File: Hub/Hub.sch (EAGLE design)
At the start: 16 parts, among them X1 C-GRID-04-15-91, X2 C-GRID-04-15-91, X3 C-GRID-04-15-91

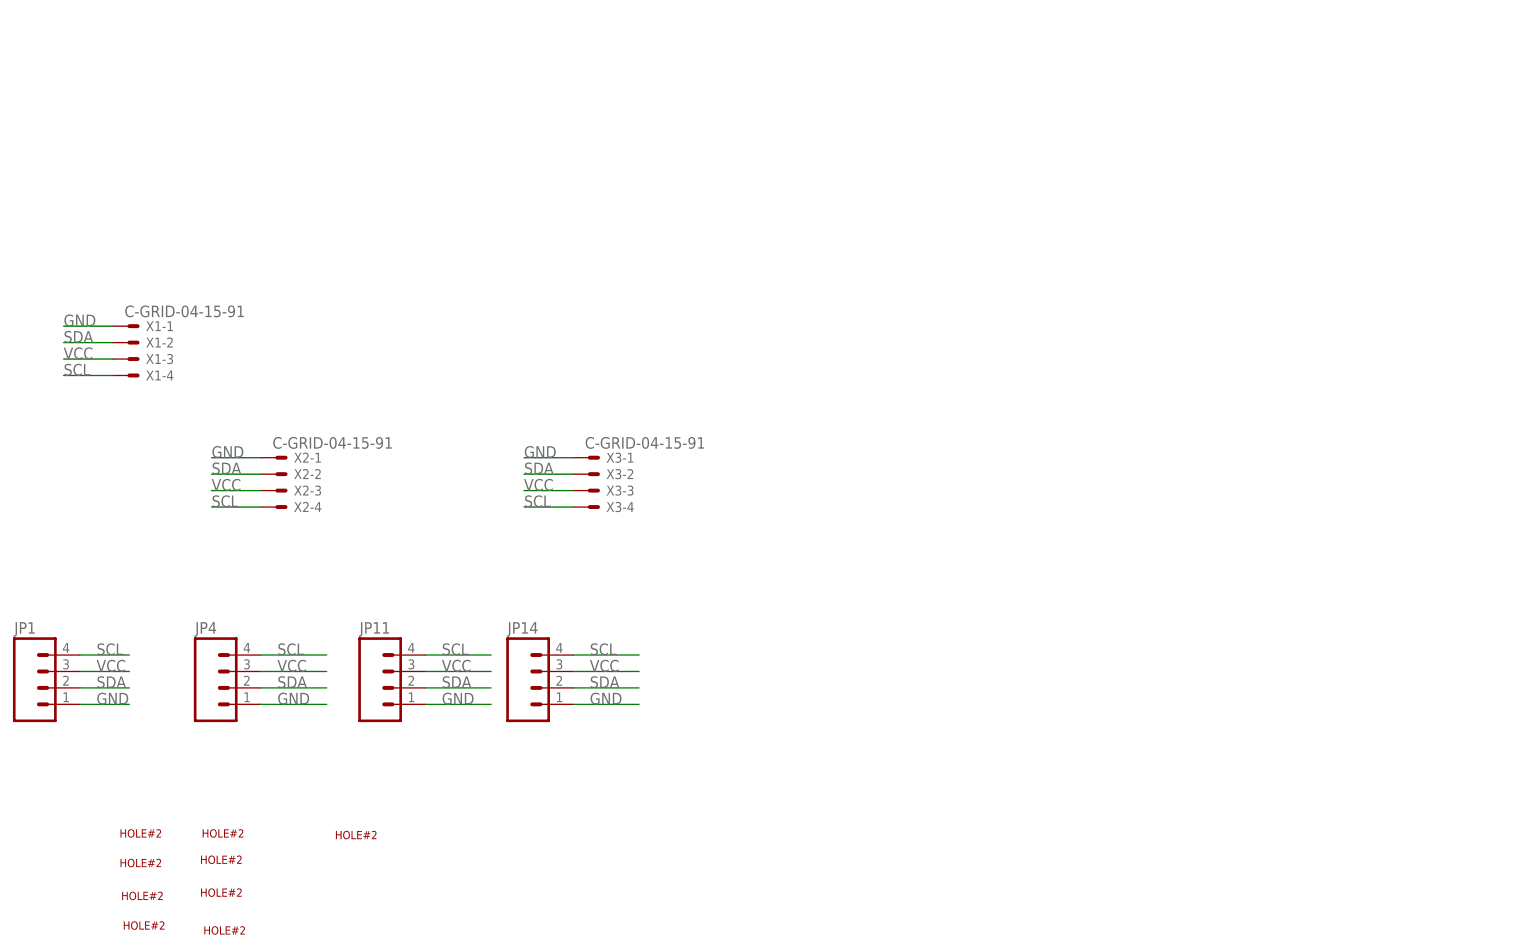
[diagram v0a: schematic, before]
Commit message: various minor changes
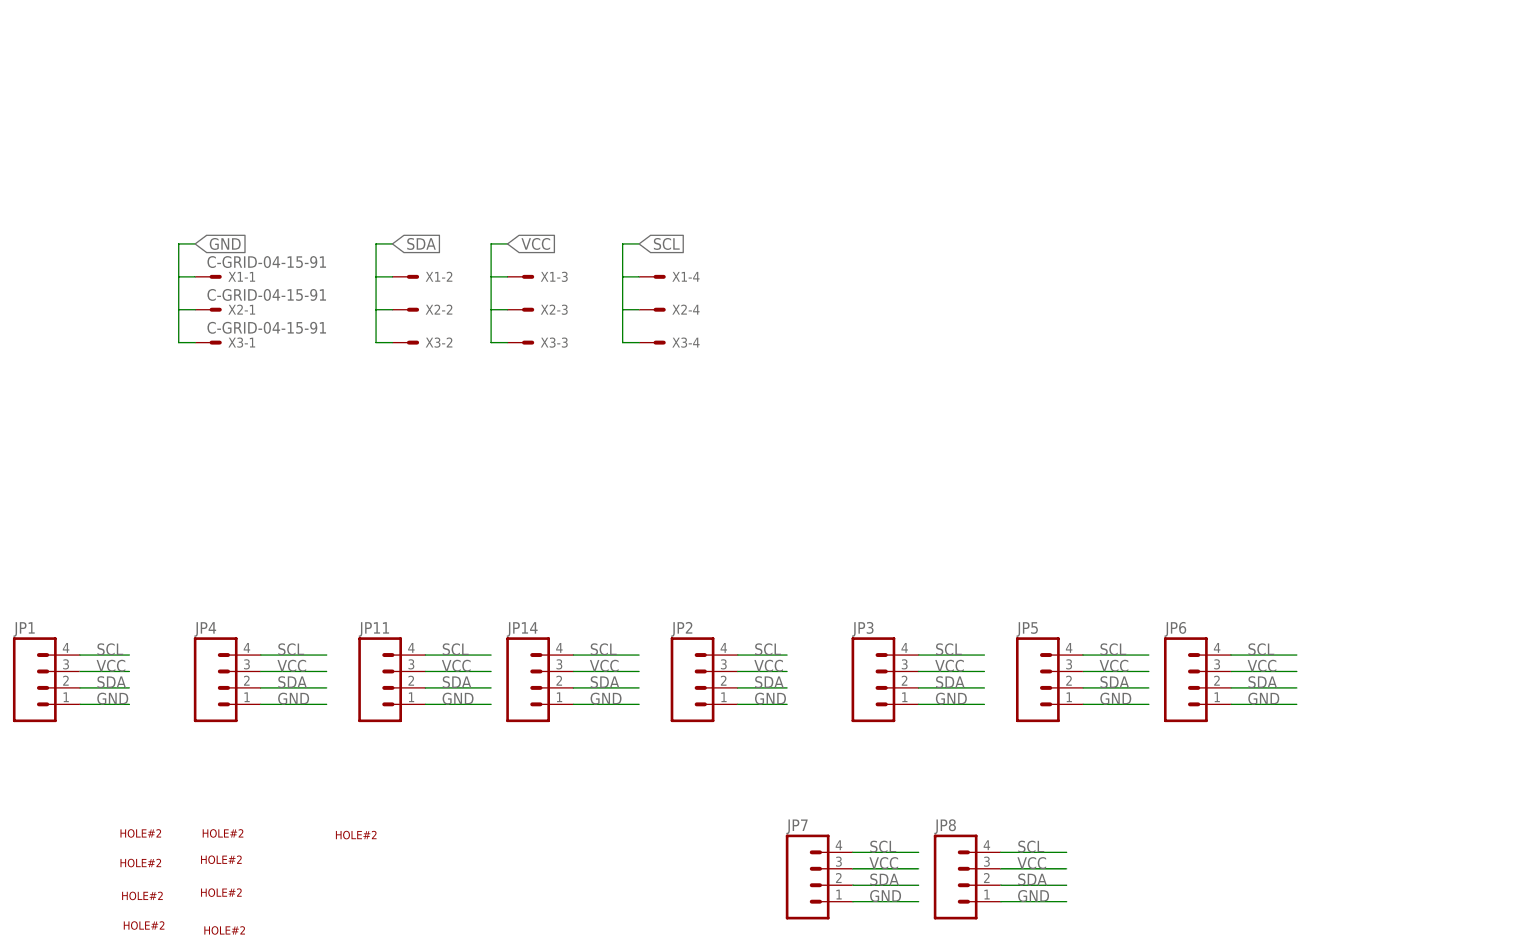
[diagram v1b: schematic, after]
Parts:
- added JP2, JP3, JP5, JP6, JP7, JP8: (no value), SparkFun-Connectors:M04LOCK
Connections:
- net GND: now also JP2.1, JP3.1, JP5.1, JP6.1, JP7.1, JP8.1
- net SCL: now also JP2.4, JP3.4, JP5.4, JP6.4, JP7.4, JP8.4
- net SDA: now also JP2.2, JP3.2, JP5.2, JP6.2, JP7.2, JP8.2
- net VCC: now also JP2.3, JP3.3, JP5.3, JP6.3, JP7.3, JP8.3
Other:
- moved on the sheet: X1-1, X1-2, X1-3, X1-4, X2-1, X2-2, X2-3, X2-4, X3-1, X3-2, X3-3, X3-4

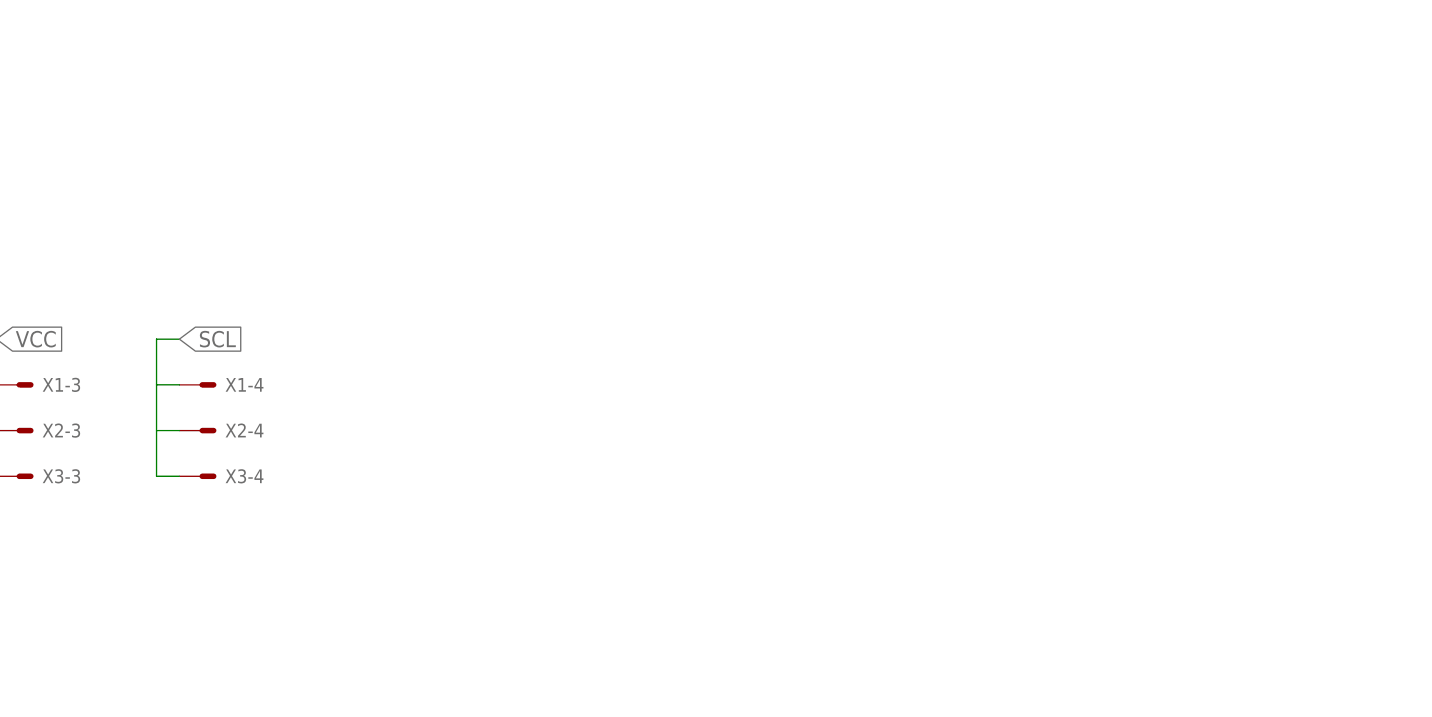
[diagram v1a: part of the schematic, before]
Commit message: Checkpointing PCB designs
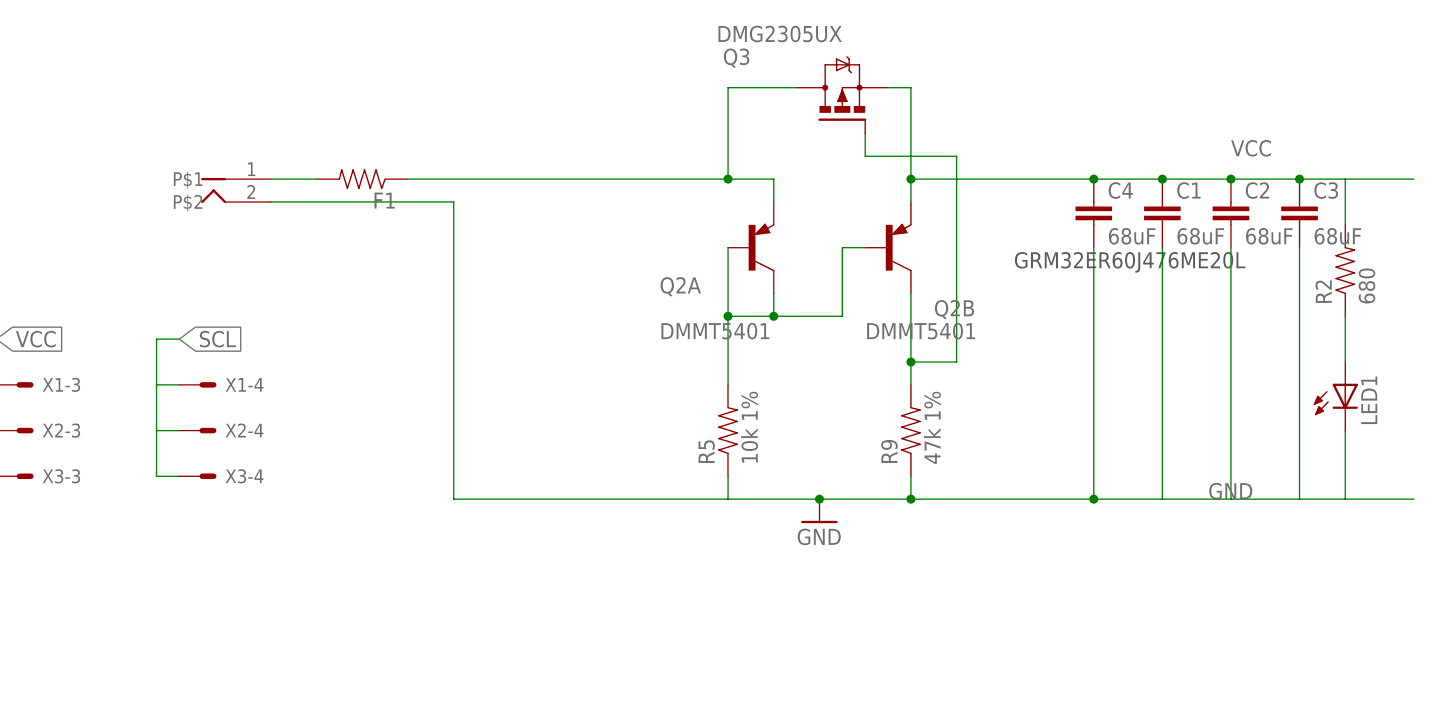
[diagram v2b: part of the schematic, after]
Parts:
- added C1, C2, C3, C4: 68uF, SparkFun-Capacitors:CAP1210
- added F1: (no value), SparkFun-Passives:RESISTOR0805-RES
- added LED1: (no value), adafruit:LEDCHIP-LED0805
- added Q2: DMMT5401, IntegerLabs:TRANSISTOR-DUAL-PNP
- added Q3: DMG2305UX, transistor-power:IRLML5203
- added R2: 680, SparkFun-Passives:RESISTOR0805-RES
- added R5: 10k 1%, SparkFun-Passives:RESISTOR0805-RES
- added R9: 47k 1%, SparkFun-Passives:RESISTOR0805-RES
- added U$1: DC-JACKLOWPRO, IntegerLabs:DC-JACKLOWPRO
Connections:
- new net N$1: F1.2, U$1.P$1
- new net N$14: Q2A.B, Q2A.C, Q2B.B, R5.2
- new net N$16: Q2B.C, Q3.G, R9.2
- new net N$8: LED1.A, R2.1
- new net VREG: F1.1, Q2A.E, Q3.D
- net GND: now also C1.2, C2.2, C3.2, C4.2, LED1.C, R5.1, R9.1, U$1.P$2
- net VCC: now also C1.1, C2.1, C3.1, C4.1, Q2B.E, Q3.S, R2.2
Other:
- note added: "GRM32ER60J476ME20L"
